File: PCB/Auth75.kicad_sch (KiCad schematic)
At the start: 209 parts, among them CN1 S2B-PH-SM4-TB, Q1 MMBT3904LT1G, Q2 MMBT3904LT1G, Q3 MMBT3904LT1G, Q4 MMBT3906LT1G, Q5 FS8205A_C2830320, SW1 EC11E15244G1, U1 RASPBERRY PI PICO 2W, U2 SL2.1S, U3 DW01A_C351410, U4 MCP73831T-2ACI/OT, U5 PCA9536DGKR

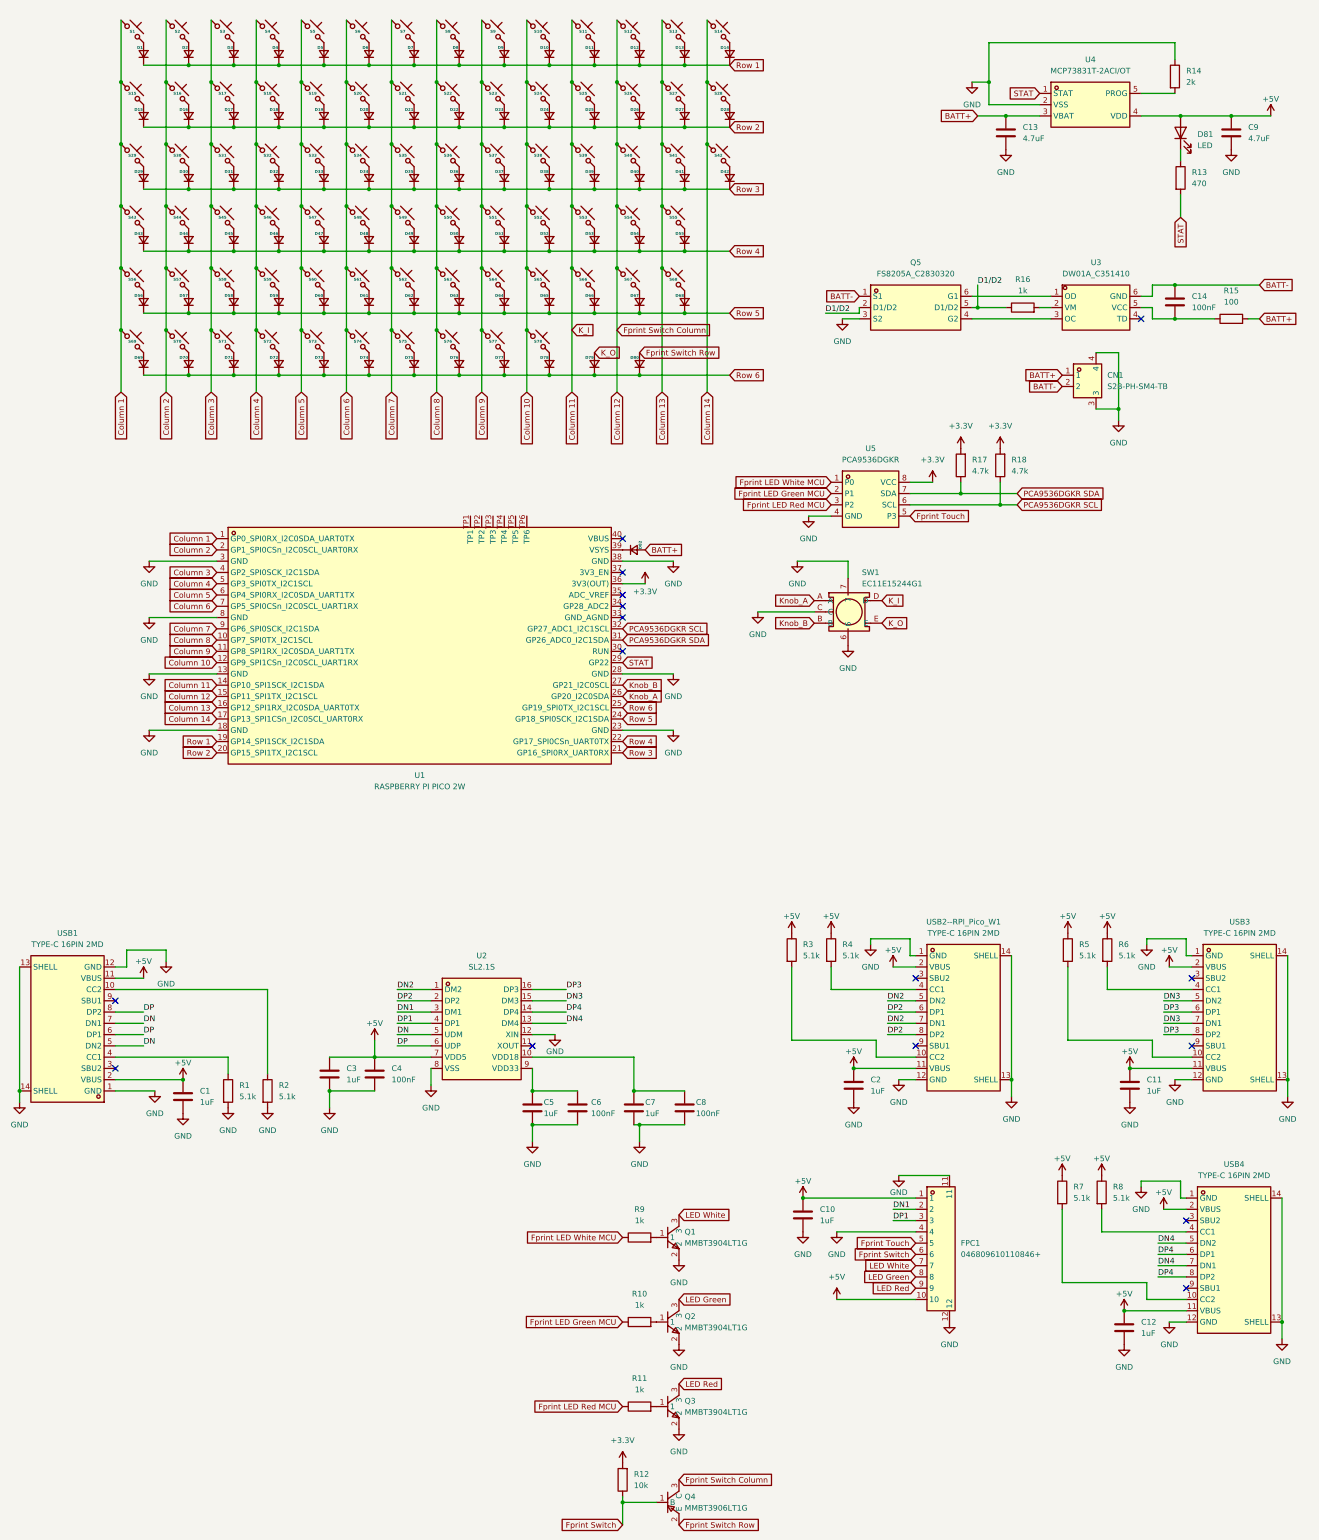
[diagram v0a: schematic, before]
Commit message: generating new CAD
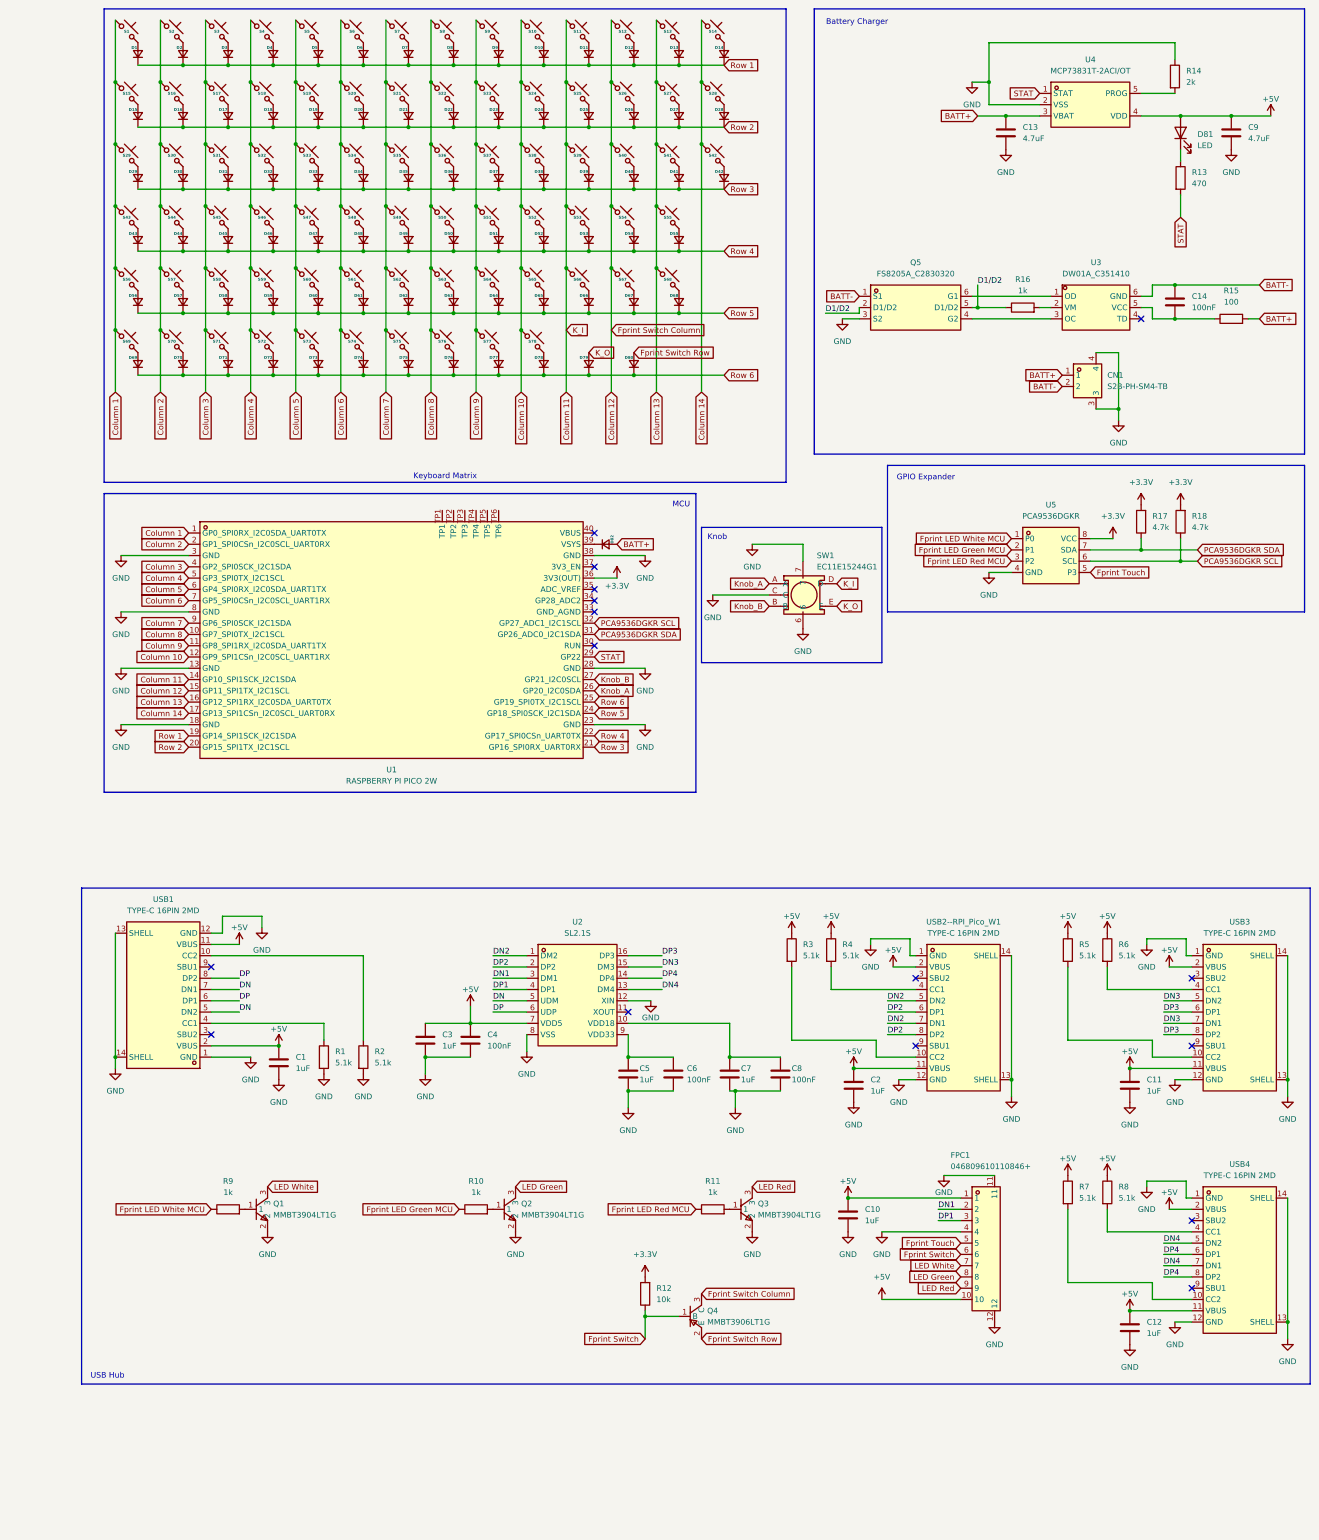
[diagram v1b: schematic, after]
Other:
- note added: "Battery Charger"
- note added: "GPIO Expander"
- note added: "Keyboard Matrix"
- note added: "Knob"
- note added: "MCU"
- note added: "USB Hub"
- moved on the sheet: C1, C10, C12, C3, C4, C5, C6, C7, C8, D1, D10, D11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
